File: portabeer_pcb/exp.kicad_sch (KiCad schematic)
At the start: 13 parts, among them J4 I2C expansion, U12 PCA9536DP, U13 GBI7254MMAR, U16 MCP47FEB12, U17 REF3012

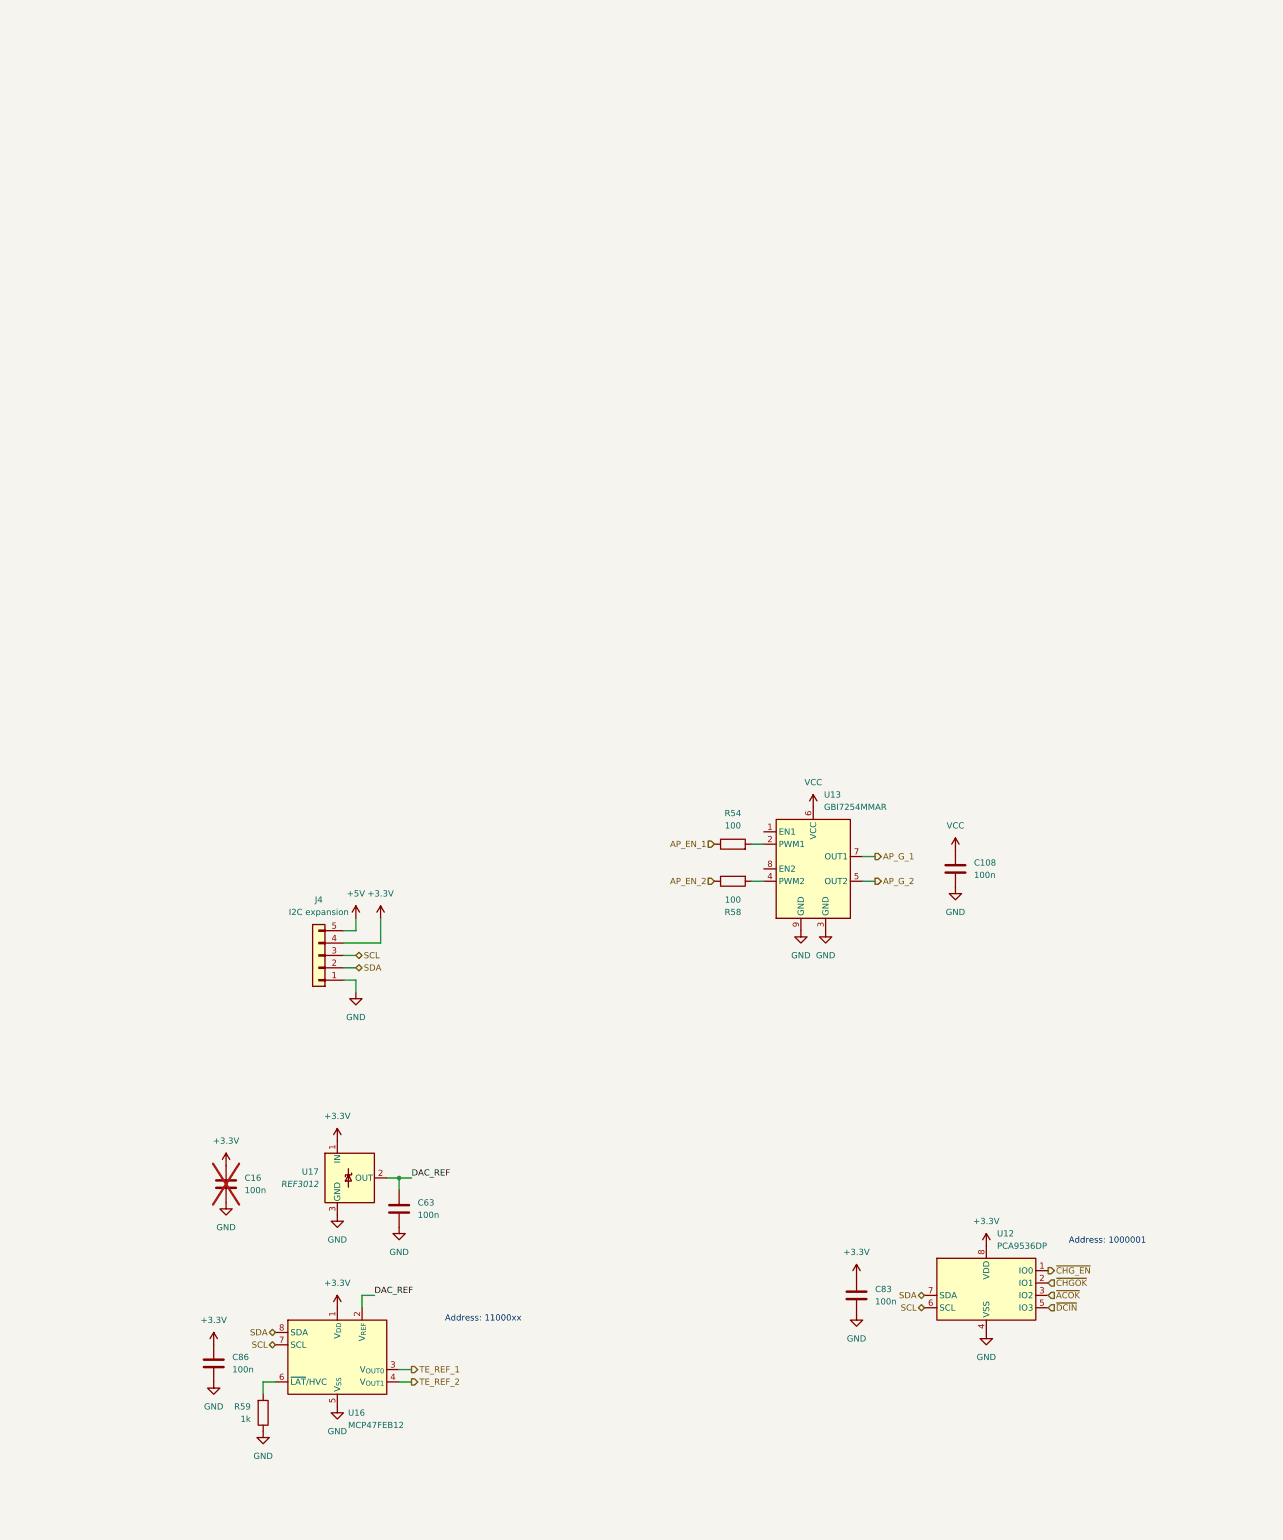
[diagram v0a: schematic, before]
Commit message: partial routing
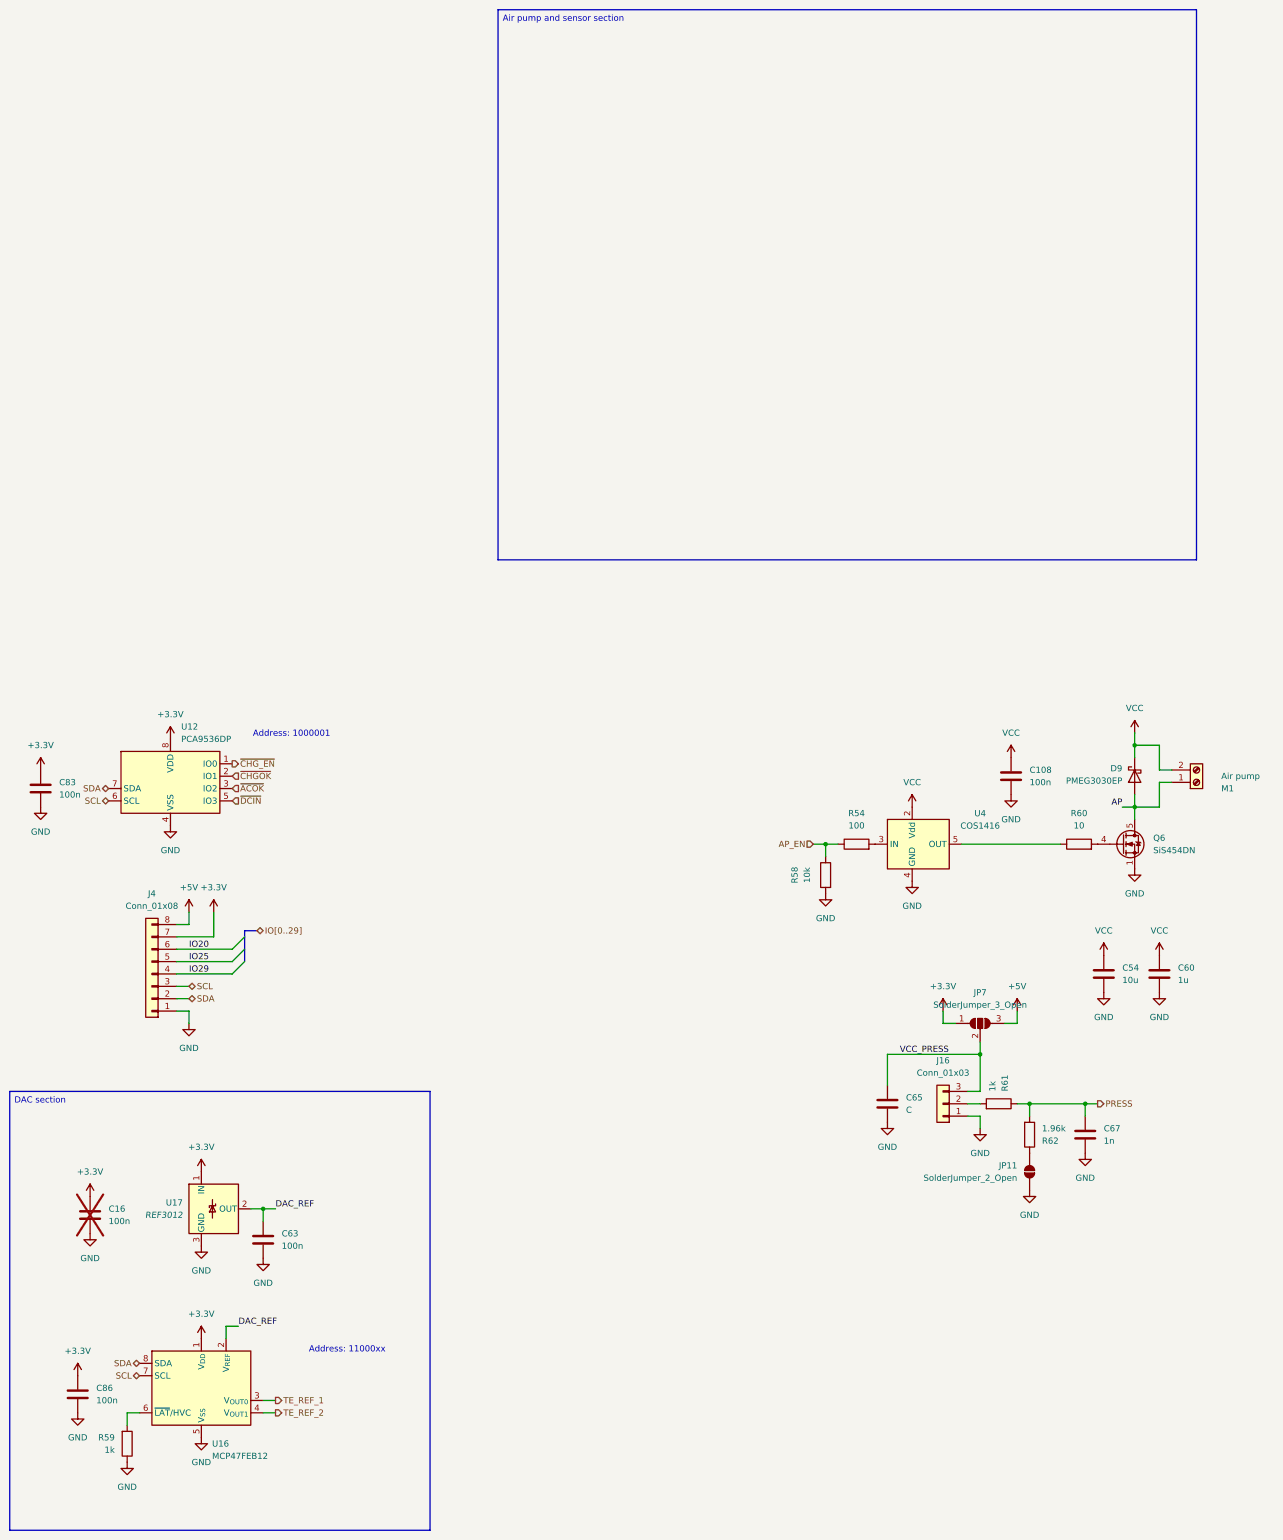
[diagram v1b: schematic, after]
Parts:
- removed J4: I2C expansion, Connector_PinHeader_2.54mm:PinHeader_1x05_P2.54mm_Vertical, symbol Connector_Generic:Conn_01x05
- removed U13: GBI7254MMAR, Package_SO:MSOP-8-1EP_3x3mm_P0.65mm_EP1.95x2.15mm, symbol Driver_FET:PM8834M
- added C54: 10u, Capacitor_SMD:C_1206_3216Metric, symbol Device:C
- added C60: 1u, Capacitor_SMD:C_0603_1608Metric, symbol Device:C
- added C65: C, Capacitor_SMD:C_0603_1608Metric, symbol Device:C
- added C67: 1n, Capacitor_SMD:C_0603_1608Metric, symbol Device:C
- added D9: PMEG3030EP, Diode_SMD:D_SOD-128, symbol Device:D_Schottky
- added J16: Conn_01x03, Connector_JST:JST_XH_B3B-XH-A_1x03_P2.50mm_Vertical, symbol Connector_Generic:Conn_01x03
- added J4: Conn_01x08, Connector_PinHeader_2.54mm:PinHeader_1x08_P2.54mm_Vertical, symbol Connector_Generic:Conn_01x08
- added JP11: SolderJumper_2_Open, Jumper:SolderJumper-2_P1.3mm_Open_RoundedPad1.0x1.5mm, symbol Jumper:SolderJumper_2_Open
- added JP7: SolderJumper_3_Open, Jumper:SolderJumper-3_P1.3mm_Open_RoundedPad1.0x1.5mm, symbol Jumper:SolderJumper_3_Open
- added M1: Air pump, Connector_Phoenix_MC:PhoenixContact_MC_1,5_2-G-3.81_1x02_P3.81mm_Horizontal, symbol Connector:Screw_Terminal_01x02
- added Q6: SiS454DN, portabeer:Vishay_PowerPAK_1212-8_Single, symbol Transistor_FET:SiS454DN
- added R60: 10, Resistor_SMD:R_0603_1608Metric, symbol Device:R
- added R61: 1k, Resistor_SMD:R_0603_1608Metric, symbol Device:R
- added R62: 1.96k, Resistor_SMD:R_0603_1608Metric, symbol Device:R
- added U4: COS1416, Package_TO_SOT_SMD:SOT-23-5, symbol Driver_FET:MCP1416
- R58: value 100 -> 10k
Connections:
- net AP_EN_2 is gone; now on net AP_EN: R58.1
- net +3.3V: now also J4.7 (Pin_7), JP7.1 (A)
- net +5V: now also J4.8 (Pin_8), JP7.3 (B)
- net GND: now also R58.2, C54.2, C60.2, C65.2, C67.2, J16.1 (Pin_1), J4.1 (Pin_1), JP11.1 (A), Q6.1 (S), Q6.2 (S), Q6.3 (S), U4.4 (GND)
- net SCL: now also J4.3 (Pin_3)
- net SDA: now also J4.2 (Pin_2)
- net VCC: now also C54.1, C60.1, D9.1 (K), M1.2 (Pin_2), U4.2 (Vdd)
- net at R54.2: now also U4.3 (IN)
- net AP_EN_1 renamed AP_EN
- new net: JP11.2 (B), R62.1
- new net: R60.1, U4.5 (OUT)
- new net: J16.2 (Pin_2), R61.2
- new net: Q6.4 (G), R60.2
- new net AP: D9.2 (A), M1.1 (Pin_1), Q6.5 (D)
- new net IO20: J4.6 (Pin_6)
- new net IO25: J4.5 (Pin_5)
- new net IO29: J4.4 (Pin_4)
- new net PRESS: C67.1, R61.1, R62.2
- new net VCC_PRESS: C65.1, J16.3 (Pin_3), JP7.2 (C)
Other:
- moved on the sheet: C108, C16, C63, C83, C86, R54, R58, R59, U12, U16, U17
